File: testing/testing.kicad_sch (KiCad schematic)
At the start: 6 parts

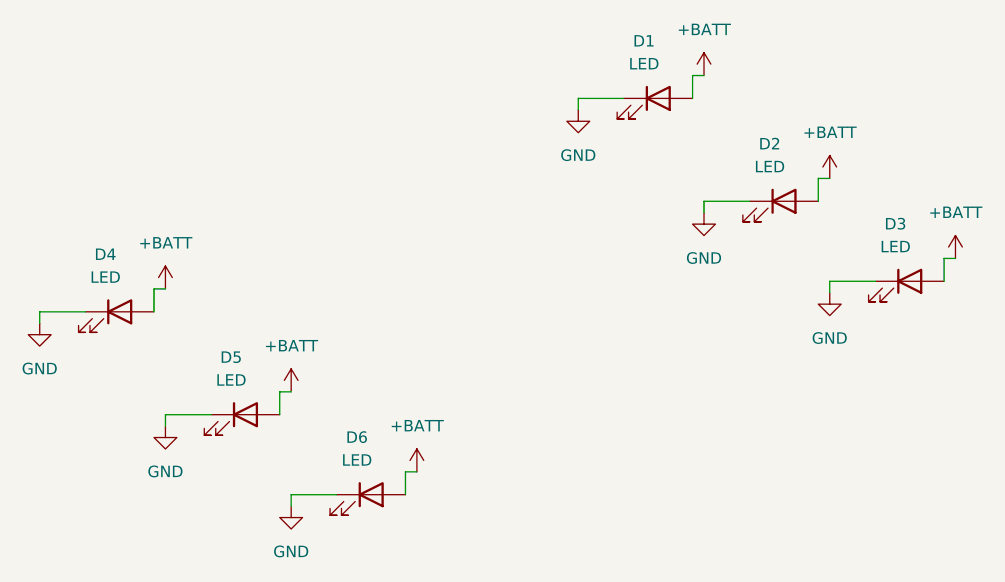
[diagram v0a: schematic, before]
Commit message: Test Commit 11
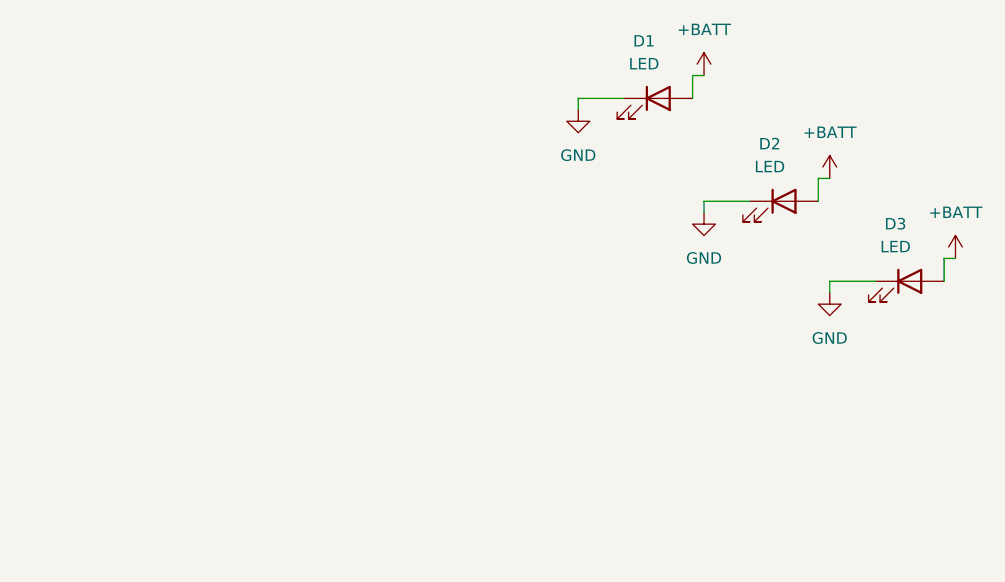
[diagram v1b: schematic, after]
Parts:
- removed D4, D5, D6: LED, symbol Device:LED
